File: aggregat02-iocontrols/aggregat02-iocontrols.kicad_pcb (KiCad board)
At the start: 2 copper layers, 45.7 x 101.9 mm, 75 parts, among them Q2 Q_NPN_BEC

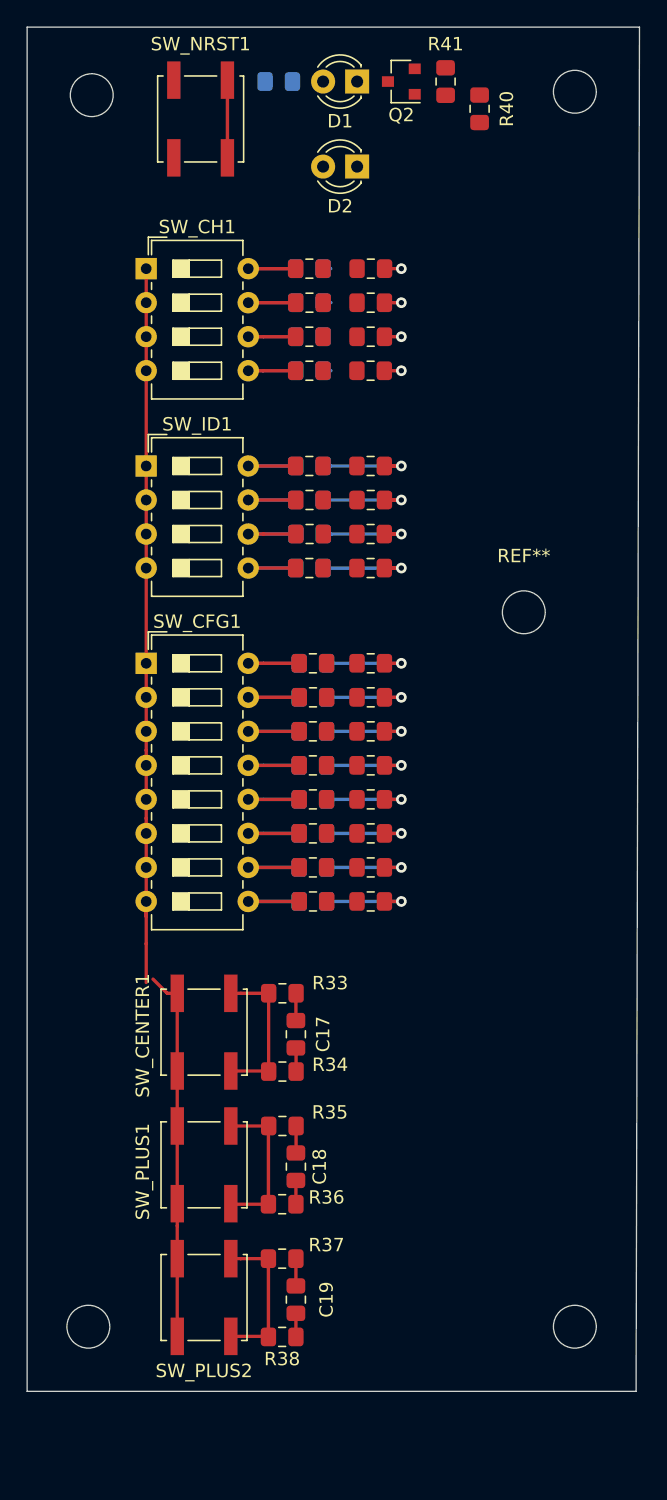
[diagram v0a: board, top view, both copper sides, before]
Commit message: v1.0"
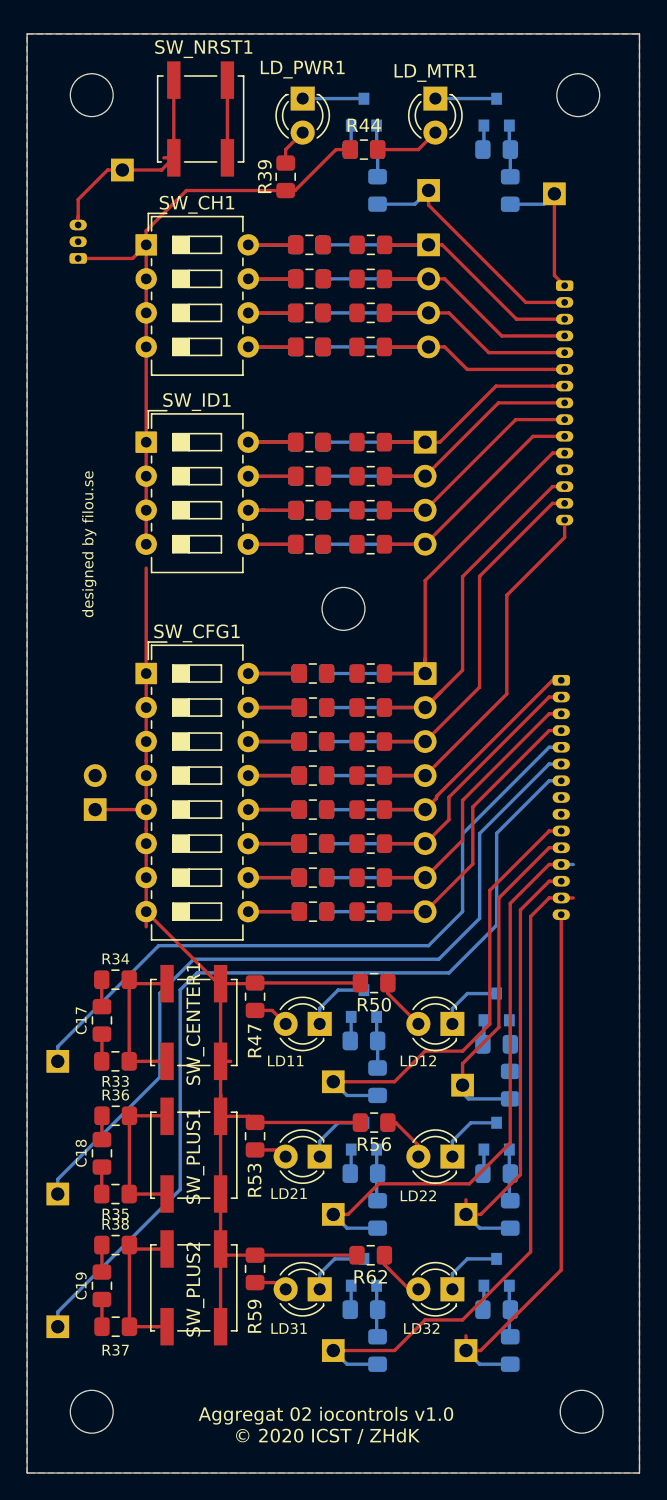
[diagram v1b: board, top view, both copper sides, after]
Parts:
- removed D2: LED, LED_THT:LED_D3.0mm
- added J1: Conn_01x04, Connector_PinHeader_2.54mm:PinHeader_1x04_P2.54mm_Vertical, B.Cu at (78.7, 69.3)
- added J10: Conn_01x01, Connector_PinHeader_2.54mm:PinHeader_1x01_P2.54mm_Vertical, B.Cu at (81.5, 117.3)
- added J11: Conn_01x01, Connector_PinHeader_2.54mm:PinHeader_1x01_P2.54mm_Vertical, B.Cu at (71.9, 127.0)
- added J12: Conn_01x01, Connector_PinHeader_2.54mm:PinHeader_1x01_P2.54mm_Vertical, B.Cu at (81.8, 127.0)
- added J13: Conn_01x01, Connector_PinHeader_2.54mm:PinHeader_1x01_P2.54mm_Vertical, B.Cu at (71.9, 137.2)
- added J14: Conn_01x01, Connector_PinHeader_2.54mm:PinHeader_1x01_P2.54mm_Vertical, B.Cu at (81.8, 137.2)
- added J15: Conn_01x15, Connector_Molex:Molex_PicoBlade_53047-1510_1x15_P1.25mm_Vertical, B.Cu at (89.2, 57.7)
- added J16: Conn_01x15, Connector_Molex:Molex_PicoBlade_53047-1510_1x15_P1.25mm_Vertical, B.Cu at (88.9, 87.1)
- added J17: Conn_01x03, Connector_PinHeader_2.54mm:PinHeader_1x02_P2.54mm_Vertical, B.Cu at (54.1, 96.8)
- added J18: Conn_01x03, Connector_Molex:Molex_PicoBlade_53047-0310_1x03_P1.25mm_Vertical, B.Cu at (52.8, 55.6)
- added J19: Conn_01x01, Connector_PinHeader_2.54mm:PinHeader_1x01_P2.54mm_Vertical, B.Cu at (56.1, 49.0)
- added J2: Conn_01x04, Connector_PinHeader_2.54mm:PinHeader_1x04_P2.54mm_Vertical, B.Cu at (79.0, 54.6)
- added J3: Conn_01x08, Connector_PinHeader_2.54mm:PinHeader_1x08_P2.54mm_Vertical, B.Cu at (78.7, 86.6)
- added J4: Conn_01x01, Connector_PinHeader_2.54mm:PinHeader_1x01_P2.54mm_Vertical, B.Cu at (51.3, 115.6)
- added J5: Conn_01x01, Connector_PinHeader_2.54mm:PinHeader_1x01_P2.54mm_Vertical, B.Cu at (51.3, 125.5)
- added J6: Conn_01x01, Connector_PinHeader_2.54mm:PinHeader_1x01_P2.54mm_Vertical, B.Cu at (51.3, 135.4)
- added J7: Conn_01x01, Connector_PinHeader_2.54mm:PinHeader_1x01_P2.54mm_Vertical, B.Cu at (79.0, 50.5)
- added J8: Conn_01x01, Connector_PinHeader_2.54mm:PinHeader_1x01_P2.54mm_Vertical, B.Cu at (88.4, 50.8)
- added J9: Conn_01x01, Connector_PinHeader_2.54mm:PinHeader_1x01_P2.54mm_Vertical, B.Cu at (71.9, 117.1)
- added LD11: LED, LED_THT:LED_D3.0mm, F.Cu at (70.9, 112.8)
- added LD12: LED, LED_THT:LED_D3.0mm, F.Cu at (80.8, 112.8)
- added LD21: LED, LED_THT:LED_D3.0mm, F.Cu at (70.9, 122.7)
- added LD22: LED, LED_THT:LED_D3.0mm, F.Cu at (80.8, 122.7)
- added LD31: LED, LED_THT:LED_D3.0mm, F.Cu at (70.9, 132.6)
- added LD32: LED, LED_THT:LED_D3.0mm, F.Cu at (80.8, 132.6)
- added LD_MTR1: LED, LED_THT:LED_D3.0mm, F.Cu at (79.5, 43.7)
- added Q1: Q_NPN_BEC, Package_TO_SOT_SMD:SOT-23, B.Cu at (84.1, 44.7)
- added Q3: Q_NPN_BEC, Package_TO_SOT_SMD:SOT-23, B.Cu at (74.2, 111.3)
- added Q4: Q_NPN_BEC, Package_TO_SOT_SMD:SOT-23, B.Cu at (84.1, 111.5)
- added Q5: Q_NPN_BEC, Package_TO_SOT_SMD:SOT-23, B.Cu at (74.2, 121.2)
- added Q6: Q_NPN_BEC, Package_TO_SOT_SMD:SOT-23, B.Cu at (84.1, 121.2)
- added Q7: Q_NPN_BEC, Package_TO_SOT_SMD:SOT-23, B.Cu at (74.2, 131.3)
- added Q8: Q_NPN_BEC, Package_TO_SOT_SMD:SOT-23, B.Cu at (84.1, 131.3)
- added R42: R 47k 1% 1/8, Resistor_SMD:R_0805_2012Metric_Pad1.15x1.40mm_HandSolder, B.Cu at (85.1, 50.6)
- added R43: R 100k 1% 1/8, Resistor_SMD:R_0805_2012Metric_Pad1.15x1.40mm_HandSolder, B.Cu at (84.1, 47.5)
- added R44: R 270 1% 1/8, Resistor_SMD:R_0805_2012Metric_Pad1.15x1.40mm_HandSolder, F.Cu at (74.2, 47.5)
- added R45: R 47k 1% 1/8, Resistor_SMD:R_0805_2012Metric_Pad1.15x1.40mm_HandSolder, B.Cu at (75.2, 117.1)
- added R46: R 100k 1% 1/8, Resistor_SMD:R_0805_2012Metric_Pad1.15x1.40mm_HandSolder, B.Cu at (74.2, 114.0)
- added R47: R 270 1% 1/8, Resistor_SMD:R_0805_2012Metric_Pad1.15x1.40mm_HandSolder, F.Cu at (66.0, 110.7)
- added R48: R 47k 1% 1/8, Resistor_SMD:R_0805_2012Metric_Pad1.15x1.40mm_HandSolder, B.Cu at (85.1, 117.3)
- added R49: R 100k 1% 1/8, Resistor_SMD:R_0805_2012Metric_Pad1.15x1.40mm_HandSolder, B.Cu at (84.1, 114.3)
- added R50: R 270 1% 1/8, Resistor_SMD:R_0805_2012Metric_Pad1.15x1.40mm_HandSolder, F.Cu at (74.9, 109.7)
- added R51: R 47k 1% 1/8, Resistor_SMD:R_0805_2012Metric_Pad1.15x1.40mm_HandSolder, B.Cu at (75.2, 127.0)
- added R52: R 100k 1% 1/8, Resistor_SMD:R_0805_2012Metric_Pad1.15x1.40mm_HandSolder, B.Cu at (74.2, 124.0)
- added R53: R 270 1% 1/8, Resistor_SMD:R_0805_2012Metric_Pad1.15x1.40mm_HandSolder, F.Cu at (66.0, 121.2)
- added R54: R 47k 1% 1/8, Resistor_SMD:R_0805_2012Metric_Pad1.15x1.40mm_HandSolder, B.Cu at (85.1, 127.0)
- added R55: R 100k 1% 1/8, Resistor_SMD:R_0805_2012Metric_Pad1.15x1.40mm_HandSolder, B.Cu at (84.1, 124.0)
- added R56: R 270 1% 1/8, Resistor_SMD:R_0805_2012Metric_Pad1.15x1.40mm_HandSolder, F.Cu at (74.9, 120.1)
- added R57: R 47k 1% 1/8, Resistor_SMD:R_0805_2012Metric_Pad1.15x1.40mm_HandSolder, B.Cu at (75.2, 137.2)
- added R58: R 100k 1% 1/8, Resistor_SMD:R_0805_2012Metric_Pad1.15x1.40mm_HandSolder, B.Cu at (74.2, 134.1)
- added R59: R 270 1% 1/8, Resistor_SMD:R_0805_2012Metric_Pad1.15x1.40mm_HandSolder, F.Cu at (66.0, 131.1)
- added R60: R 47k 1% 1/8, Resistor_SMD:R_0805_2012Metric_Pad1.15x1.40mm_HandSolder, B.Cu at (85.1, 137.2)
- added R61: R 100k 1% 1/8, Resistor_SMD:R_0805_2012Metric_Pad1.15x1.40mm_HandSolder, B.Cu at (84.1, 134.1)
- added R62: R 270 1% 1/8, Resistor_SMD:R_0805_2012Metric_Pad1.15x1.40mm_HandSolder, F.Cu at (74.7, 130.0)
- Q2, R41: moved to B.Cu
- R39: value R -> R 270 1% 1/8; moved to F.Cu
- R40: value R 270 1% 1/8 -> R 47k 1% 1/8; moved to B.Cu
- moved REF** 37.4 mm to (90.4, 141.7)
- moved REF** 36.6 mm to (53.8, 141.7)
- moved C17 14.5 mm to (54.6, 112.5), turned to 90 degrees
- moved C19 14.5 mm to (54.6, 132.3), turned to 90 degrees
- moved C18 14.5 mm to (54.6, 122.4), turned to 90 degrees
- moved R34 14.2 mm to (55.6, 109.5), turned to 0 degrees
- moved R38 14.2 mm to (55.6, 129.3), turned to 0 degrees
- moved R36 14.1 mm to (55.6, 119.6), turned to 0 degrees
- moved REF** 13.5 mm to (72.6, 81.8)
- moved R33 13.5 mm to (55.6, 115.6), turned to 0 degrees
- moved R35 13.5 mm to (55.6, 125.5), turned to 0 degrees
- moved R37 13.4 mm to (55.6, 135.4), turned to 0 degrees
- moved R40 9.76 mm to (75.2, 50.5)
- moved R41 7.94 mm to (74.2, 47.5), turned to 180 degrees
- moved R39 7.13 mm to (68.3, 49.5), turned to 270 degrees
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- renumbered D1 to LD_PWR1
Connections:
- R40 pad 2: LED_1 -> LED_PWR
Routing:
- net SW_PLUS2: track 2.03 -> 69.9 mm
- net +3V3: track 82.4 -> 143.7 mm
- net SW_PLUS1: track 2.02 -> 60.9 mm
- net SW_CENTER: track 2.04 -> 53.4 mm
- net LED31: track 0.00 -> 50.3 mm
- net LED21: track 0.00 -> 42.9 mm
- net LED32: track 0.00 -> 41.0 mm
- net LED11: track 0.00 -> 34.3 mm
- net LED22: track 0.00 -> 33.8 mm
- net SW_CFG_4: track 6.84 -> 33.8 mm, vias 1 -> 0
- net SW_CFG_2: track 6.84 -> 33.4 mm, vias 1 -> 0
- net SW_CFG_1: track 6.84 -> 32.8 mm, vias 1 -> 0
- net LED12: track 0.00 -> 25.6 mm
- net SW_CFG_3: track 7.42 -> 33.0 mm, vias 1 -> 0
- net SW_CH_1: track 1.83 -> 23.7 mm, vias 1 -> 0
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- added copper zone on B.Cu, net GNDREF
- added copper zone on F.Cu, net GNDREF
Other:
- board size 45.7 x 101.9 mm -> 45.7 x 107.4 mm
- board text added: "Aggregat 02 iocontrols v1.0 © 2020 ICST / ZHdK"
- board text added: "designed by filou.se"
